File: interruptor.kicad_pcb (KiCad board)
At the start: 2 copper layers, 23 parts, among them J1 220v, J2 tx/rx, J3 Screw_Terminal_01x03, J4 Screw_Terminal_01x03, J5 Int_1, J6 int_2, J7 switch, K1 SRD-05VDC-SL-C, K2 SRD-05VDC-SL-C, Q1 PN2222A, Q2 PN2222A, U1 HLK-PM01, U2 LM1117-3.3, U3 ESP-07v2

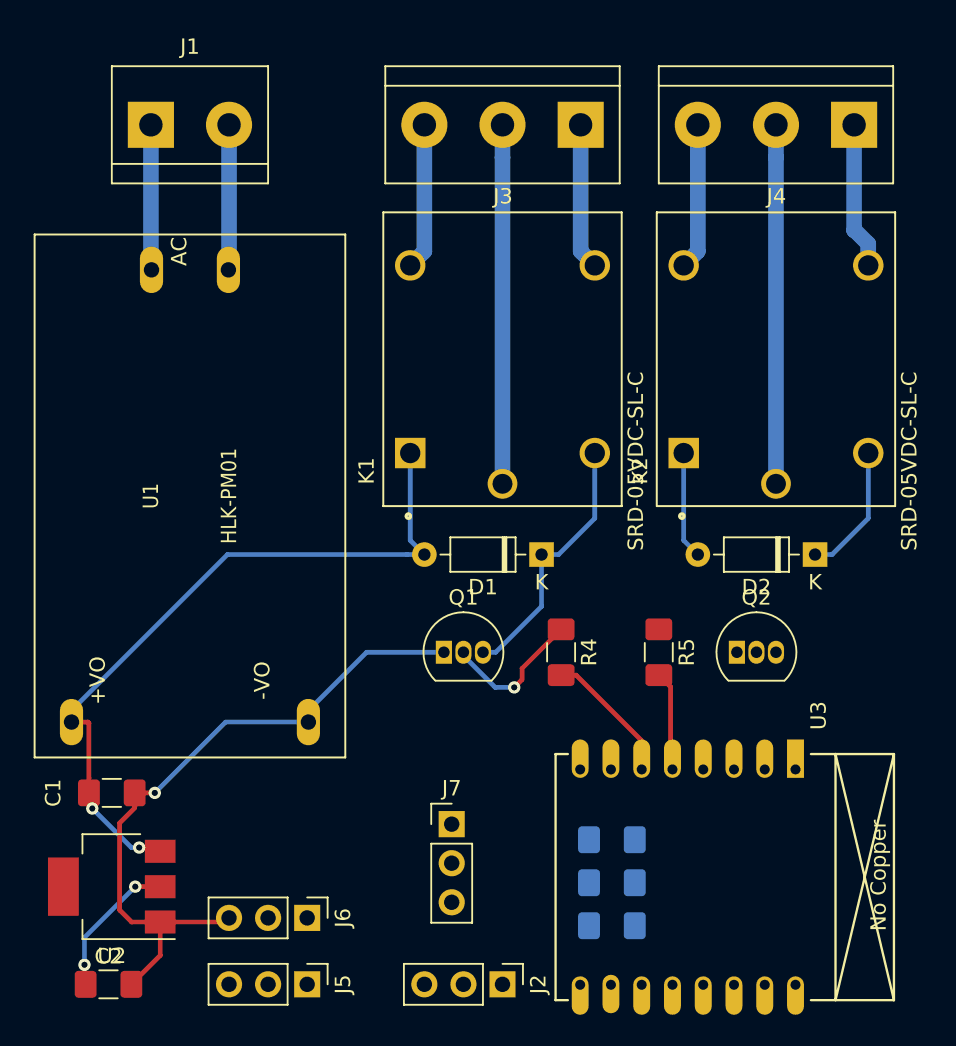
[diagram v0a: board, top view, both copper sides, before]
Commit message: pistas dibujadas
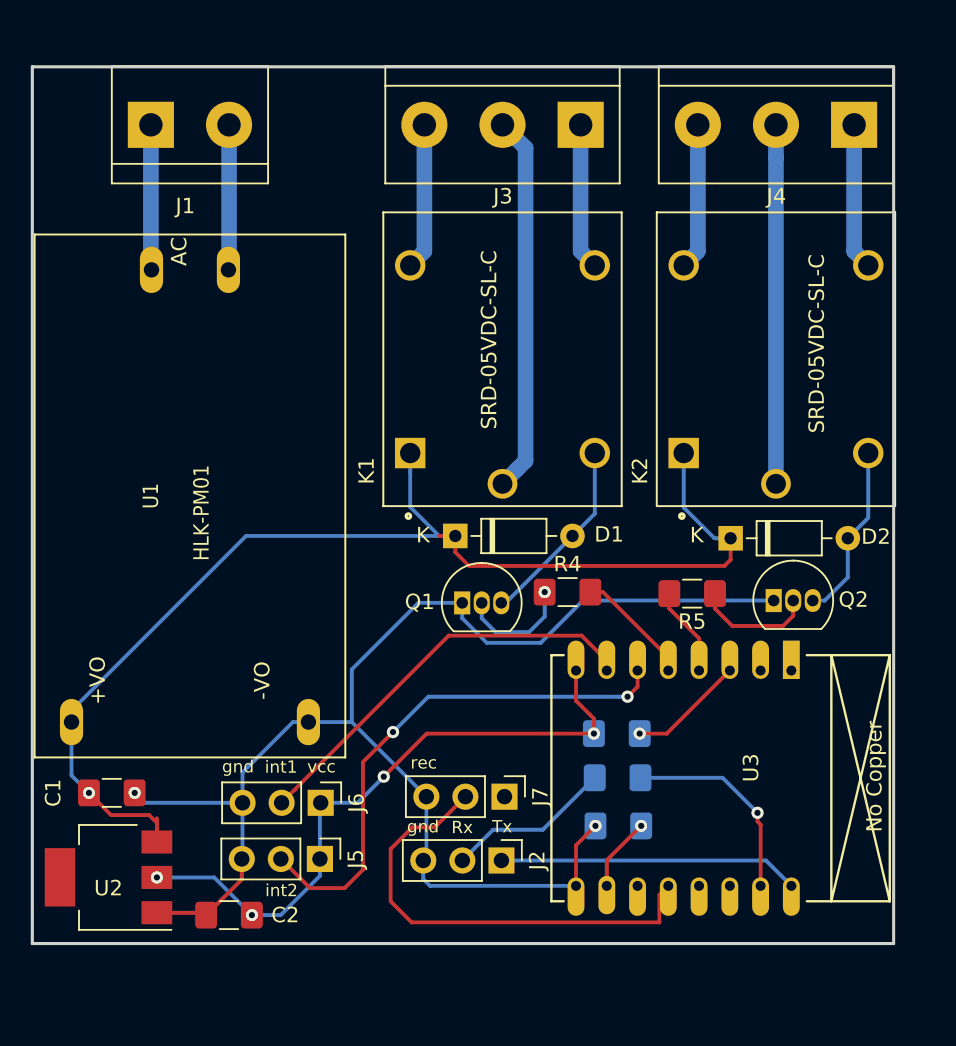
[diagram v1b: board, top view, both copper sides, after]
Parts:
- moved C2 9.04 mm to (97.8, 116.2), turned to 180 degrees
- moved J5 8.19 mm to (103.7, 112.5)
- moved J2 8.05 mm to (115.5, 112.6)
- moved J6 7.53 mm to (103.8, 108.8)
- moved R1 6.91 mm to (123.0, 104.3)
- moved R3 6.83 mm to (123.0, 107.2)
- moved R2 6.50 mm to (123.1, 110.3)
- moved U3 6.44 mm to (134.3, 100.2)
- moved D1 5.74 mm to (112.5, 91.5), turned to 0 degrees
- moved D2 5.59 mm to (130.4, 91.7), turned to 0 degrees
- moved R5 4.38 mm to (127.9, 95.2), turned to 180 degrees
- moved Q2 4.12 mm to (133.2, 95.7)
- moved R4 3.93 mm to (119.8, 95.2), turned to 0 degrees
- moved J7 3.87 mm to (115.7, 108.5), turned to 270 degrees
- moved Q1 3.42 mm to (113.0, 95.8)
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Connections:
- U3 pad 4: int_1 -> Relay_2
- U3 pad 5: Relay_2 -> Relay_1
- U3 pad 6: Relay_1 -> int_1
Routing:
- net GND: track 44.7 -> 91.5 mm, vias 1 -> 2
- net int_1: track 0.00 -> 34.6 mm, vias 0 -> 2
- net vcc: track 9.37 -> 41.6 mm, vias 2 -> 4
- net Net-(J7-Pad2): track 0.00 -> 30.3 mm
- net int_2: track 0.00 -> 27.0 mm
- net Net-(C1-Pad1): track 54.2 -> 79.0 mm
- net Net-(J2-Pad1): track 0.00 -> 19.5 mm
- net Net-(R3-Pad2): track 0.00 -> 13.4 mm, vias 0 -> 1
- net Net-(J2-Pad2): track 0.00 -> 10.8 mm
- net Net-(Q2-Pad2): track 0.00 -> 7.79 mm
- net Net-(R1-Pad1): track 0.00 -> 7.56 mm, vias 0 -> 1
- net Net-(R2-Pad1): track 0.00 -> 4.83 mm, vias 0 -> 1
- net Net-(D1-Pad1): track 17.1 -> 12.4 mm
- net Net-(D2-Pad1): track 8.68 -> 11.5 mm
- net Net-(Q1-Pad2): track 9.42 -> 7.47 mm
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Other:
- board outline added: 56 x 57 mm
- board text added: "Rx"
- board text added: "Tx"
- board text added: "gnd"
- board text added: "int1"
- board text added: "int2"
- board text added: "rec"
- board text added: "vcc"
